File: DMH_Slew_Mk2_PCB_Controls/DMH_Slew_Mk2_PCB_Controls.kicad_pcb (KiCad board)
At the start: 2 copper layers, 48 x 141 mm, 21 parts, among them J19 Conn_01x08, J20 Conn_01x08, J29 Conn_01x08, J30 Conn_01x08, SW1 SW_DPDT_3way, SW2 SW_DPDT, SW3 SPDT_OnOffOn, SW4 SW_DPDT_3way, SW5 SW_DPDT, SW6 SPDT_OnOffOn

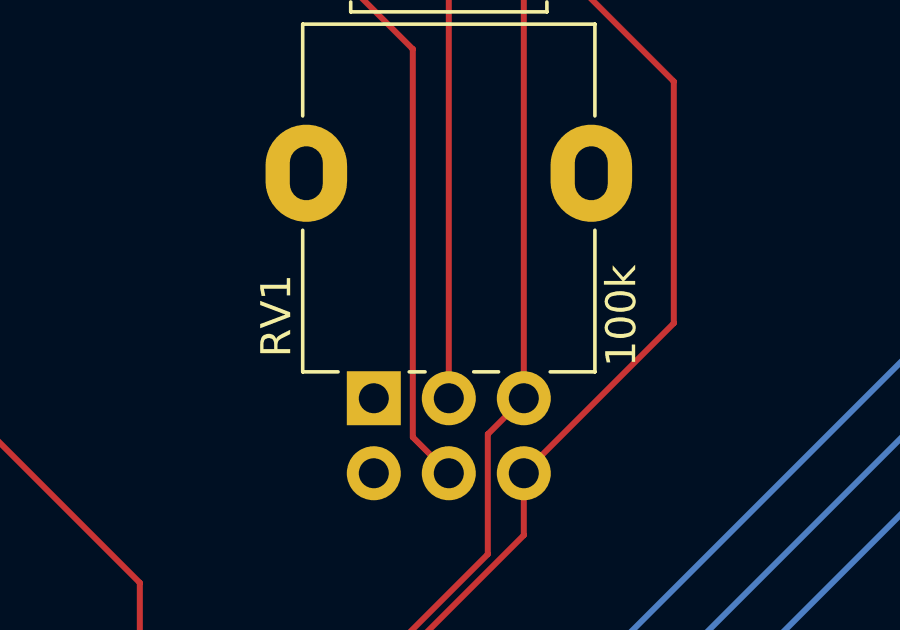
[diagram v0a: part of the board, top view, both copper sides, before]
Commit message: Updated SynthStuff
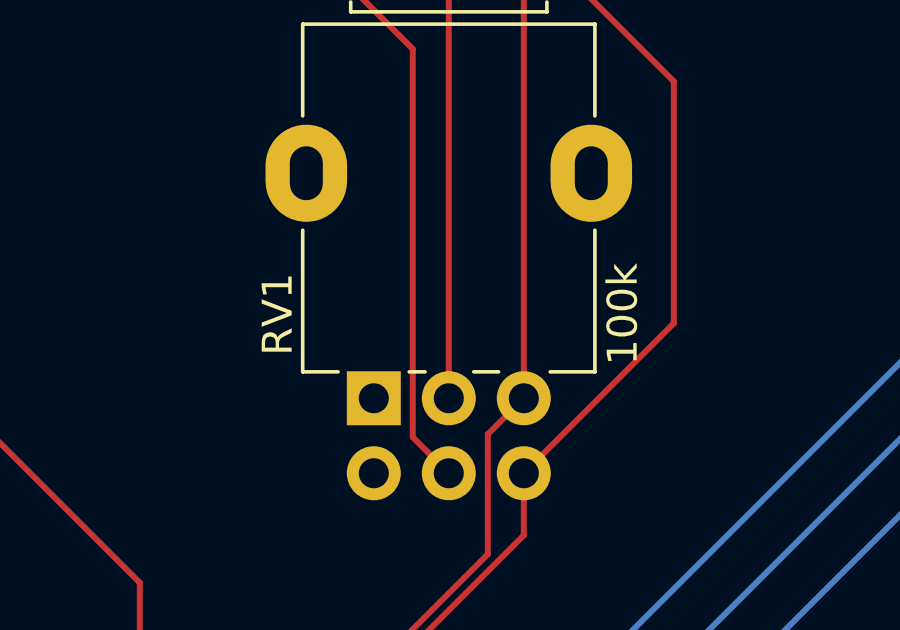
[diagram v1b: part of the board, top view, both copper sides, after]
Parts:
- RV1: footprint Potentiometer_THT:Potentiometer_Alpha_RD902F-40-00D_Dual_Vertical -> SynthStuff:Potentiometer_Alpha_RD902F-40-00D_Dual_Vertical
